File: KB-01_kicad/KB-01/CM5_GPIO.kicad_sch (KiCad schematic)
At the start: 11 parts, among them J7 Conn_01x03, SW1 Right angle Tact button, U13 74LVC1G07SE-7

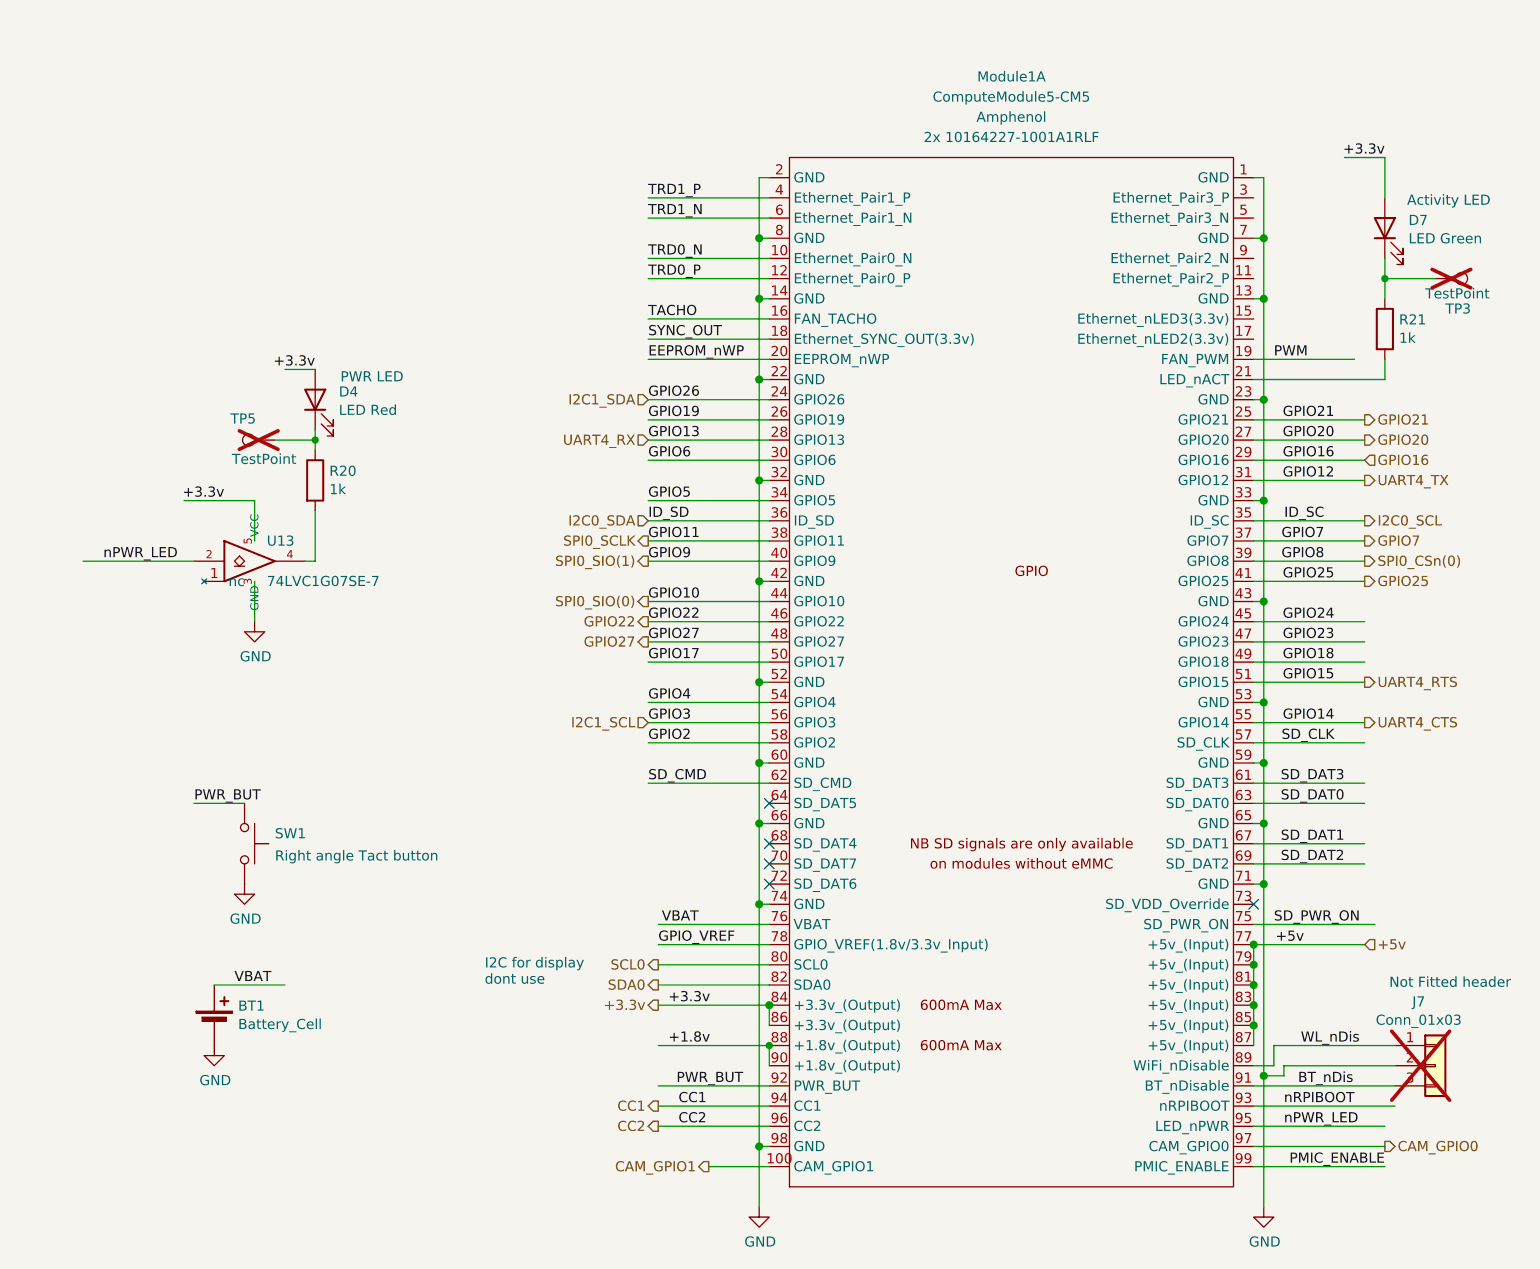
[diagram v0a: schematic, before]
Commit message: everything
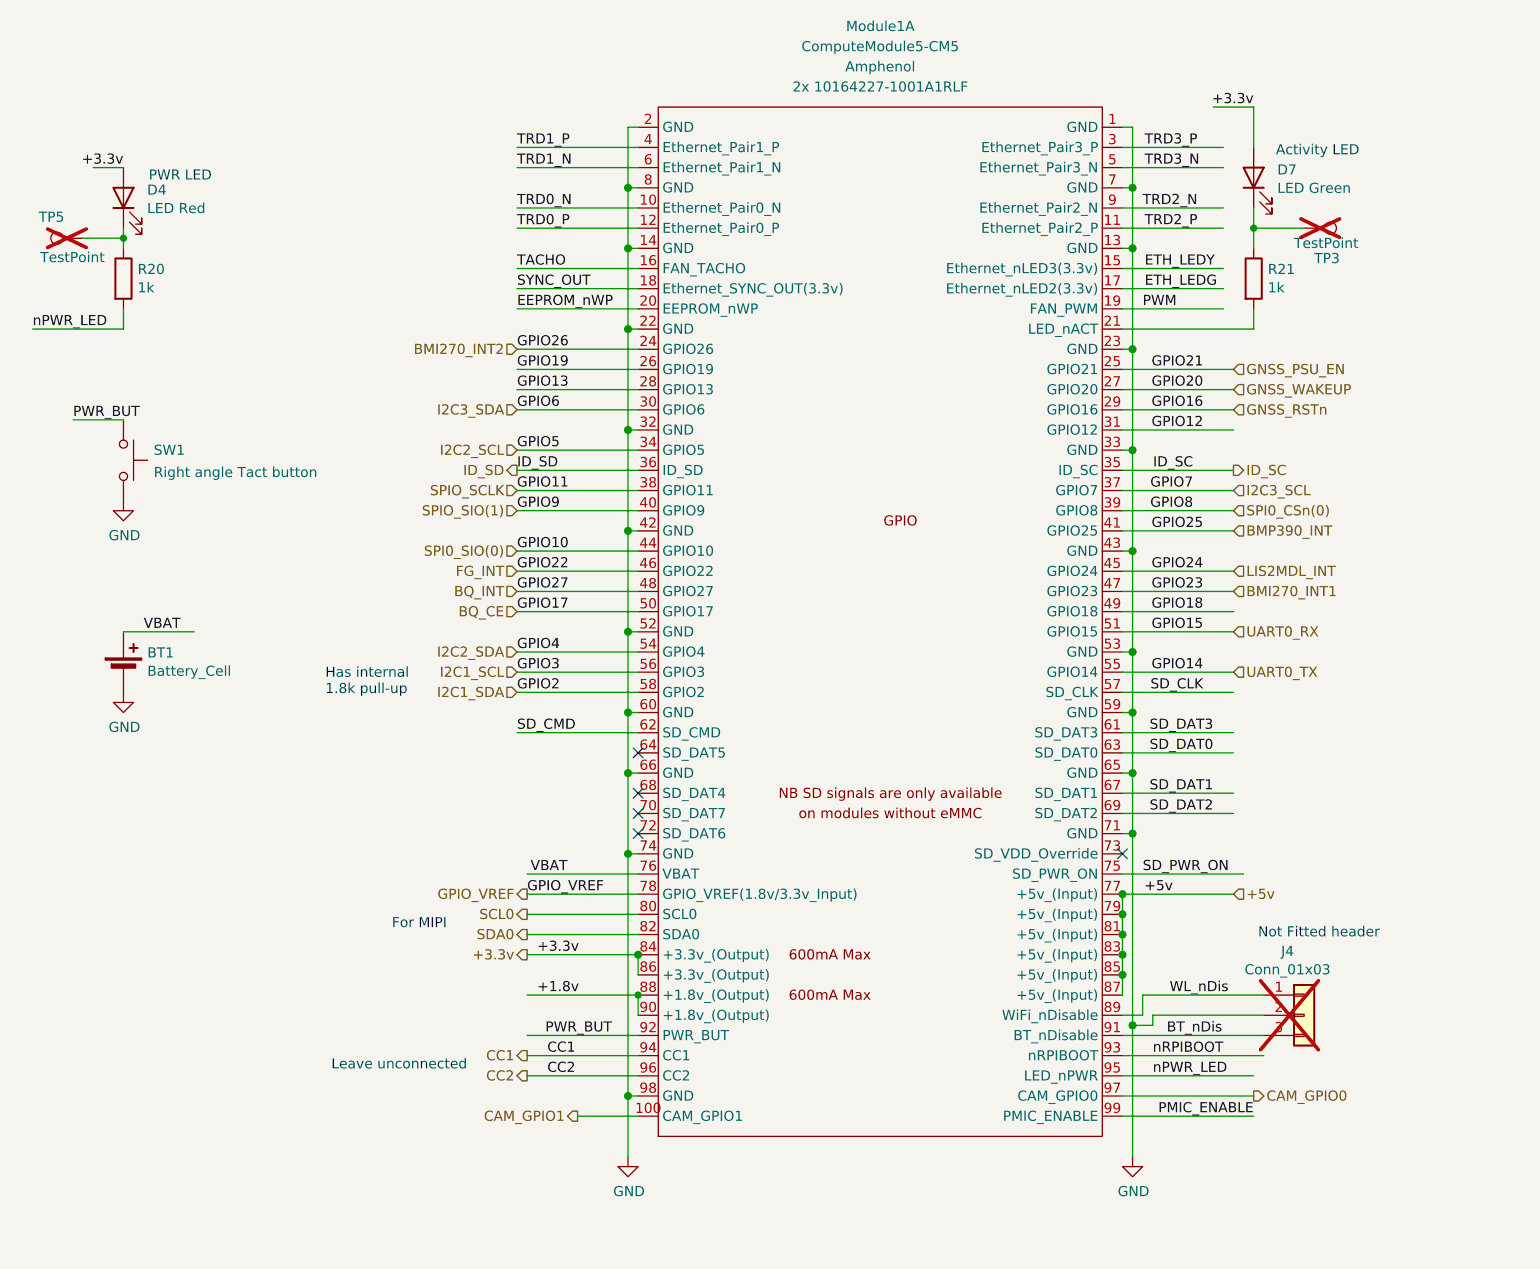
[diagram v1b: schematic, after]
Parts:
- removed J7: Conn_01x03, Connector_PinHeader_2.54mm:PinHeader_1x03_P2.54mm_Vertical, symbol Connector_Generic:Conn_01x03
- removed U13: 74LVC1G07SE-7, Package_TO_SOT_SMD:SOT-353_SC-70-5, symbol CM5IO:74LVC1G07_copy
- added J4: Conn_01x03, Connector_PinHeader_2.54mm:PinHeader_1x03_P2.54mm_Vertical, symbol Connector_Generic:Conn_01x03
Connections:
- net GPIO2 is gone; now on net I2C1_SDA: Module1.58 (GPIO2)
- net BT_nDis: now also J4.3 (Pin_3)
- net GND: now also J4.2 (Pin_2)
- net I2C1_SDA: no longer Module1.24 (GPIO26)
- net WL_nDis: now also J4.1 (Pin_1)
- net nPWR_LED: now also R20.2
- net TRD2_P: now reaches Module1.11 (Ethernet_Pair2_P)
- net ETH_LEDY: now reaches Module1.15 (Ethernet_nLED3(3.3v))
- net ETH_LEDG: now reaches Module1.17 (Ethernet_nLED2(3.3v))
- net TRD3_P: now reaches Module1.3 (Ethernet_Pair3_P)
- net TRD3_N: now reaches Module1.5 (Ethernet_Pair3_N)
- net TRD2_N: now reaches Module1.9 (Ethernet_Pair2_N)
- net GPIO16 renamed GNSS_RSTn
- net GPIO17 renamed BQ_CE
- net GPIO20 renamed GNSS_WAKEUP
- net GPIO21 renamed GNSS_PSU_EN
- net GPIO22 renamed FG_INT
- net GPIO23 renamed BMI270_INT1
- net GPIO24 renamed LIS2MDL_INT
- net GPIO25 renamed BMP390_INT
- net GPIO27 renamed BQ_INT
- net GPIO4 renamed I2C2_SDA
- net GPIO5 renamed I2C2_SCL
- net GPIO6 renamed I2C3_SDA
- net GPIO7 renamed I2C3_SCL
- net I2C0_SCL renamed ID_SC
- net I2C0_SDA renamed ID_SD
- net SPI0_SCLK renamed SPIO_SCLK
- net SPI0_SIO(1) renamed SPIO_SIO(1)
- net UART4_CTS renamed UART0_TX
- net UART4_RTS renamed UART0_RX
- net UART4_RX renamed GPIO13
- net UART4_TX renamed GPIO12
- new net BMI270_INT2: Module1.24 (GPIO26)
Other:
- note added: "For MIPI"
- note added: "Has internal 1.8k pull-up"
- note added: "Leave unconnected"
- note removed: "I2C for display dont use"
- moved on the sheet: BT1, Module1A, SW1, TP3, TP5
